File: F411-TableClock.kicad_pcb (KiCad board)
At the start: 2 copper layers, 80.7 x 76 mm, 45 parts, among them J1 USB_C_Receptacle_USB2.0_16P, J2 Conn_01x16_Socket, J3 Conn_01x04_Pin, J4 Conn_01x09_Socket, J5 Conn_01x09_Socket, Q1 DMG3415U, Q2 BC547, SW1 SW_Push, SW2 SW_Push, SW3 SW_Push, SW4 SW_Push, U1 STM32F411CCUx, U2 AP2204K-3.3, U3 AM2302, Y1 Crystal

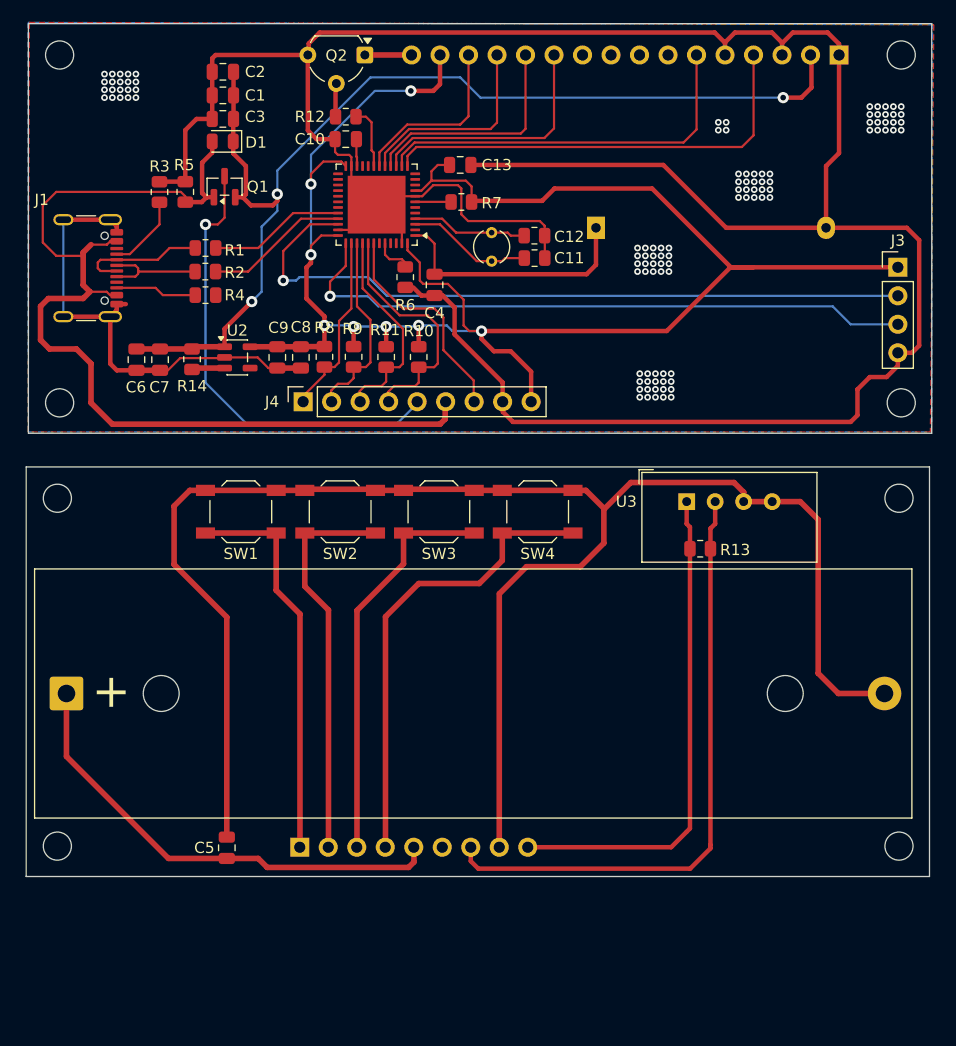
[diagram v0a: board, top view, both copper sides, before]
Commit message: Refactor code structure for improved readability and maintainability
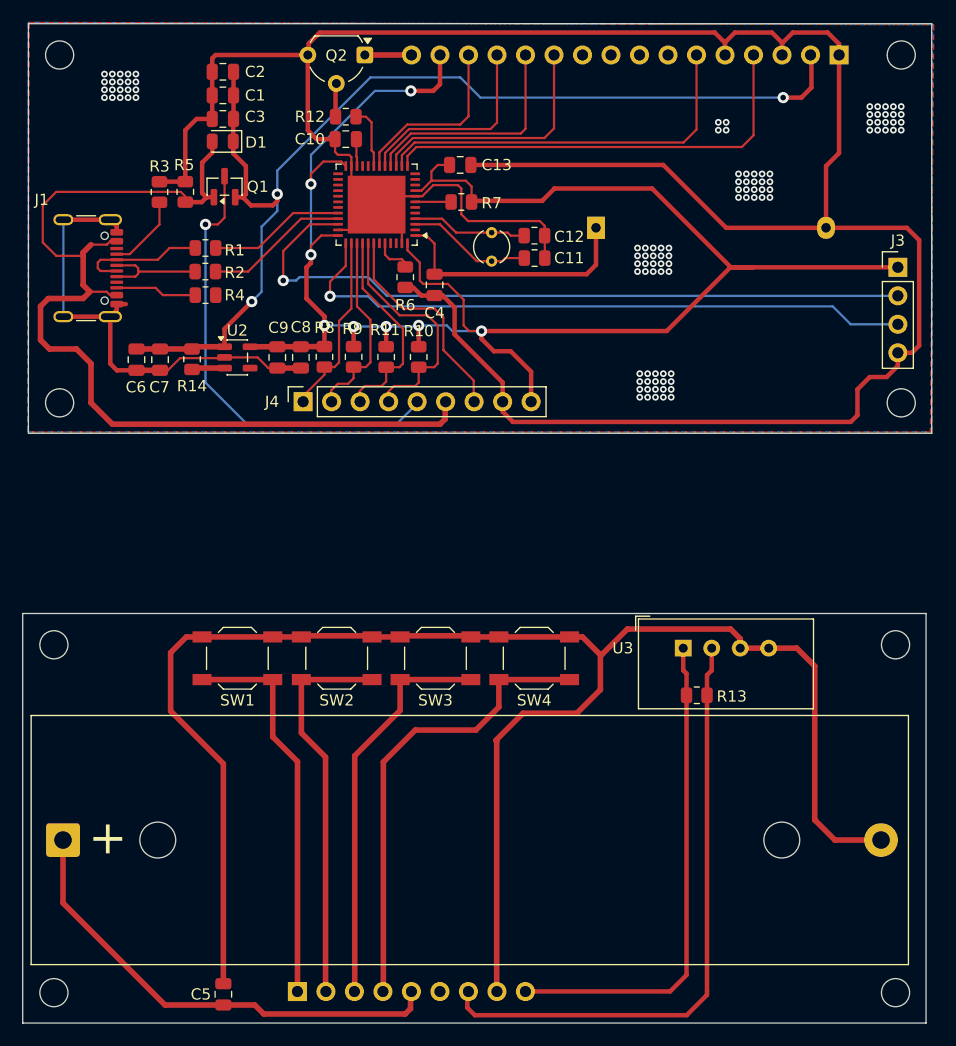
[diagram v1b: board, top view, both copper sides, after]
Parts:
- moved BT1 13.1 mm to (94.1, 122.6)
- moved C5 13.1 mm to (108.4, 136.3)
- moved R13 13.1 mm to (150.6, 109.7)
- moved SW1 13.1 mm to (109.6, 106.4)
- moved SW2 13.1 mm to (118.5, 106.4)
- moved SW3 13.1 mm to (127.3, 106.4)
- moved SW4 13.1 mm to (136.1, 106.4)
- moved U3 13.1 mm to (149.4, 105.5)
- moved J5 12.9 mm to (115.0, 136.1)
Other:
- board size 80.7 x 76 mm -> 81 x 89.1 mm
